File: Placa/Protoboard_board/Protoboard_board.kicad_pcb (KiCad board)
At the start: 2 copper layers, 40.7 x 40.9 mm, 4 parts, among them J1 Conn_02x05_Counter_Clockwise, J2 Right_Conector, J3 Left_Conector, U1 CH32V003FxPx

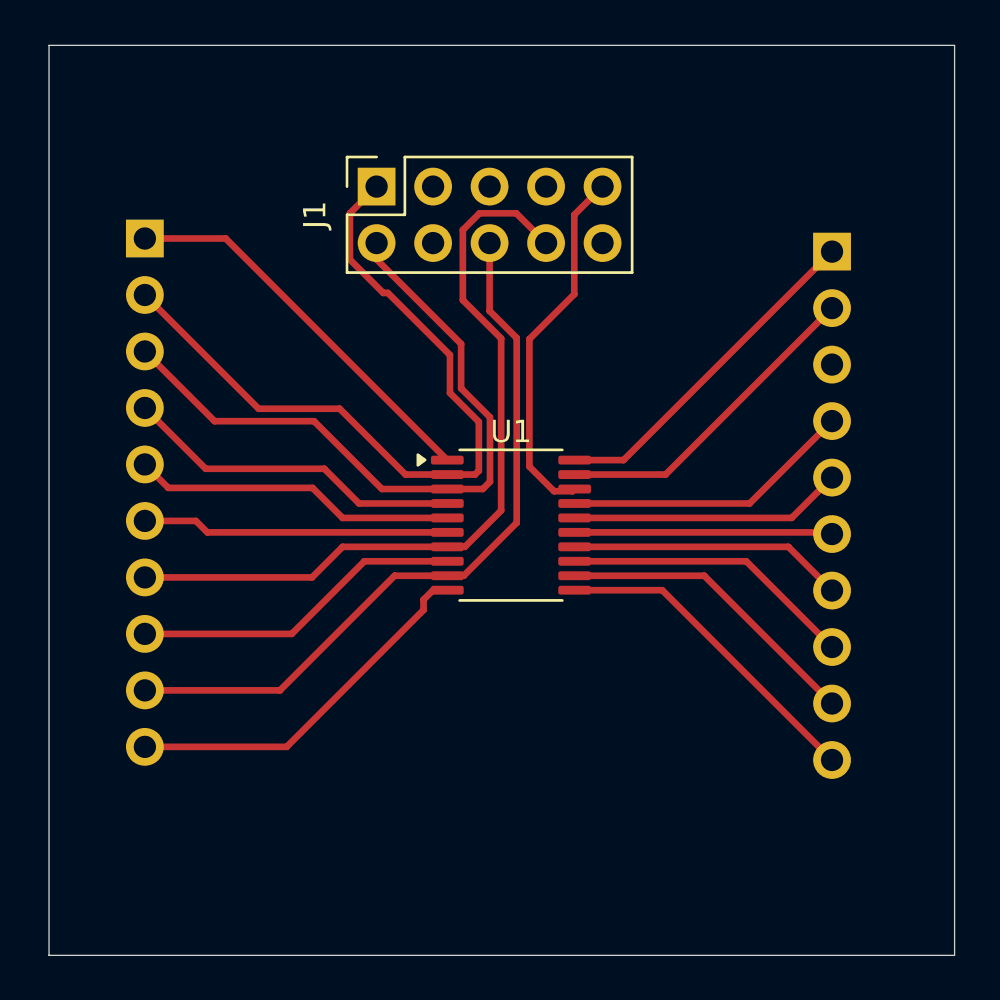
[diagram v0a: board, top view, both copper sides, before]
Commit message: Função do PWM
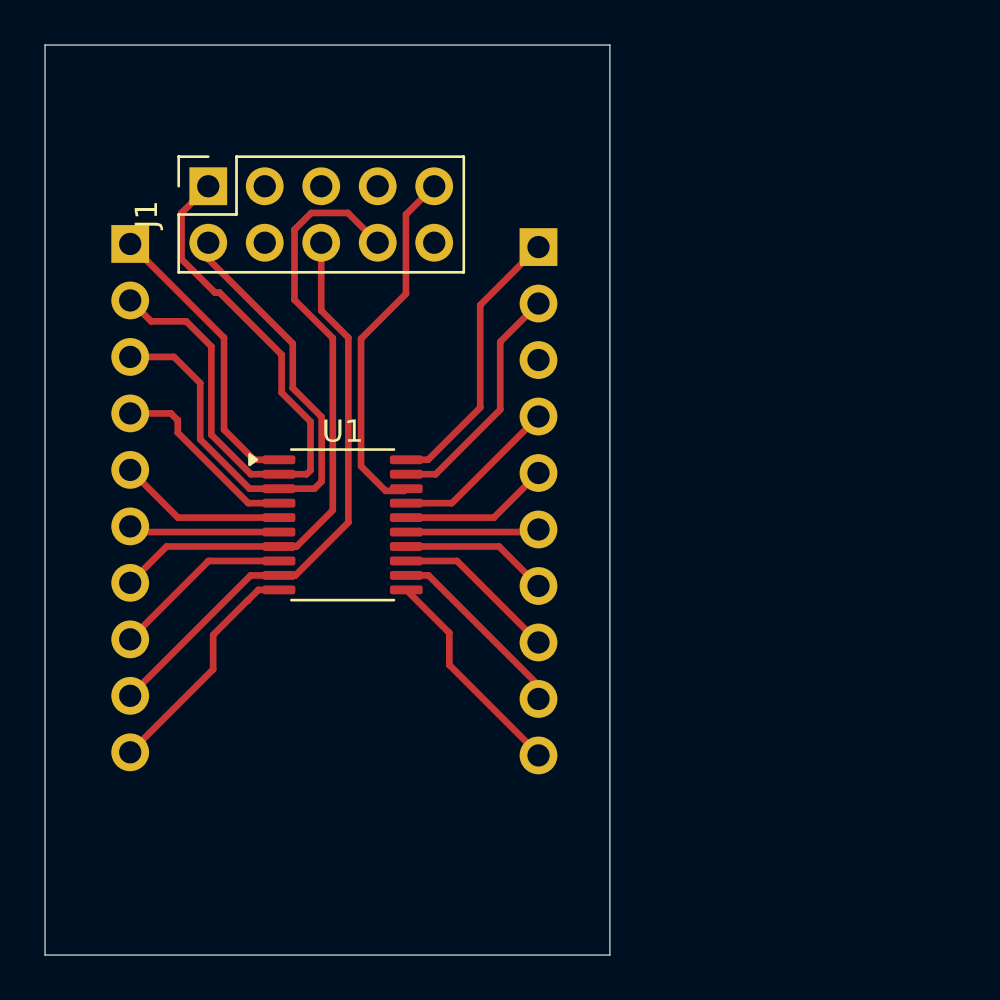
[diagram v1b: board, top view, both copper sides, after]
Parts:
- moved J2 13.2 mm to (54.7, 39.2)
- moved J1 7.57 mm to (39.8, 36.4)
- moved U1 7.57 mm to (45.9, 51.6)
- moved J3 0.70 mm to (36.3, 39.0)
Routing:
- net /PA2: track 13.8 -> 6.80 mm
- net /PA1: track 14.6 -> 7.58 mm
- net /5V_linker: track 32.9 -> 26.1 mm
- net GND: track 35.2 -> 28.4 mm
- net /PD0: track 15.0 -> 8.15 mm
- net /PD7: track 15.4 -> 8.69 mm
- net /PC0: track 16.8 -> 10.6 mm
- net /PC3: track 13.2 -> 7.46 mm
- net /PC4: track 12.4 -> 6.68 mm
- net /PC5: track 11.6 -> 5.99 mm
- net /PC7: track 13.1 -> 7.56 mm
- net /PC6: track 12.3 -> 6.78 mm
- net /PD6: track 31.1 -> 25.5 mm
- net /PC2: track 14.0 -> 8.60 mm
- net /PC1: track 14.7 -> 9.91 mm
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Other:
- board size 40.7 x 40.9 mm -> 25.4 x 40.9 mm
